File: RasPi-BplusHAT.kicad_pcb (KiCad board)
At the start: 2 copper layers, 65 x 56 mm, 11 parts, among them K1 PIN20X2, U1 EEPROM24

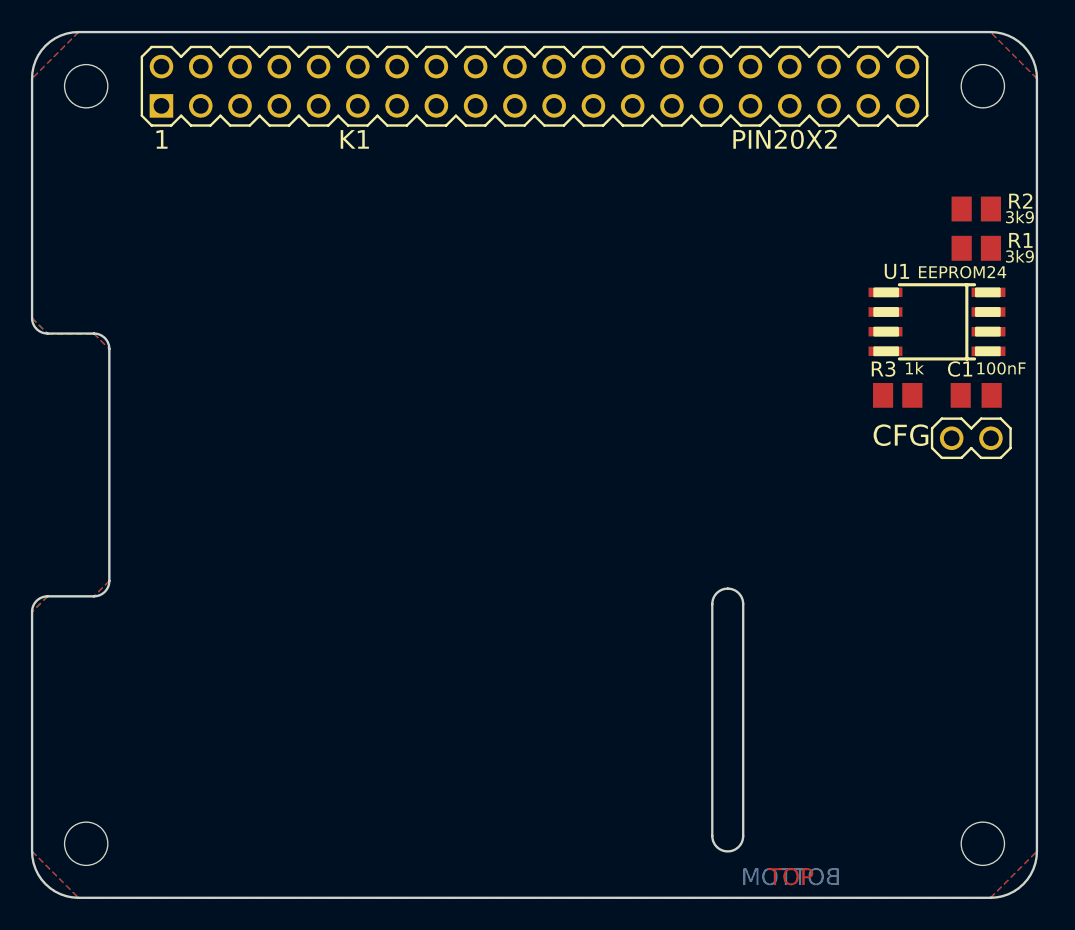
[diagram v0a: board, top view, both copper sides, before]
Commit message: Fix zones
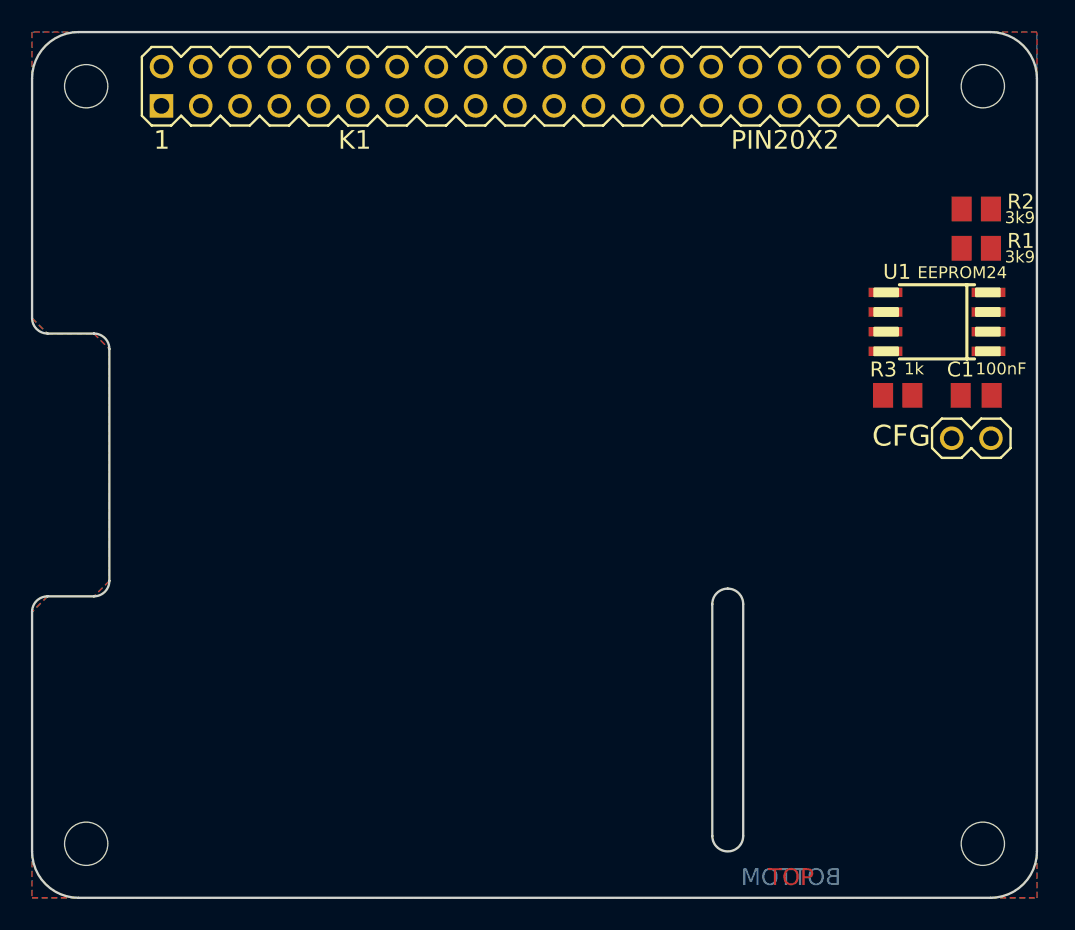
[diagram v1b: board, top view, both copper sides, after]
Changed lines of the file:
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@@
     (links 26)
     (no_connects 26)
-    (area 114.665415 76.924999 182.336786 133.075001)
+    (area 115.924999 76.924999 181.075001 133.075001)
     (thickness 1.6)
     (drawings 23)
@@
   (page A4)
   (layers
-    (0 Top signal hide)
-    (31 Bottom signal hide)
+    (0 Top signal)
+    (31 Bottom signal)
     (32 B.Adhes user)
     (33 F.Adhes user)
@@
     (42 Eco1.User user)
     (43 Eco2.User user)
-    (44 Edge.Cuts user)
+    (44 Edge.Cuts user hide)
     (45 Margin user)
     (46 B.CrtYd user)
@@
     (connect_pads (clearance 0.508))
     (min_thickness 0.254)
-    (fill (arc_segments 32) (thermal_gap 0.508) (thermal_bridge_width 0.508))
+    (fill yes (arc_segments 32) (thermal_gap 0.508) (thermal_bridge_width 0.508))
     (polygon
       (pts
-        (xy 116.0011 130.0036) (xy 119.0011 133.0036) (xy 178.0011 133.0036) (xy 181.0011 130.0036) (xy 181.0011 80.0036)
-        (xy 178.0011 77.0036) (xy 119.0011 77.0036) (xy 116.0011 80.0036) (xy 116.0011 95.5036) (xy 117.0011 96.5036)
+        (xy 116.0011 130.0036) (xy 116 133) (xy 178.0011 133.0036) (xy 181 133) (xy 181.0011 80.0036)
+        (xy 181 77) (xy 116 77) (xy 116.0011 80.0036) (xy 116.0011 95.5036) (xy 117.0011 96.5036)
         (xy 120.0011 96.5036) (xy 121.0011 97.5036) (xy 121.0011 112.5036) (xy 120.0011 113.5036) (xy 117.0011 113.5036)
         (xy 116.0011 114.5036)
@@
     (connect_pads (clearance 0.508))
     (min_thickness 0.254)
-    (fill (arc_segments 32) (thermal_gap 0.508) (thermal_bridge_width 0.508))
+    (fill yes (arc_segments 32) (thermal_gap 0.508) (thermal_bridge_width 0.508))
     (polygon
       (pts
-        (xy 116.0011 130.0036) (xy 119.0011 133.0036) (xy 178.0011 133.0036) (xy 181.0011 130.0036) (xy 181.0011 80.0036)
-        (xy 178.0011 77.0036) (xy 119.0011 77.0036) (xy 116.0011 80.0036) (xy 116.0011 95.5036) (xy 117.0011 96.5036)
+        (xy 116 133) (xy 119.0011 133.0036) (xy 181 133) (xy 181 130) (xy 181 77)
+        (xy 178.0011 77.0036) (xy 119.0011 77.0036) (xy 116 77) (xy 116.0011 95.5036) (xy 117.0011 96.5036)
         (xy 120.0011 96.5036) (xy 121.0011 97.5036) (xy 121.0011 112.5036) (xy 120.0011 113.5036) (xy 117.0011 113.5036)
         (xy 116.0011 114.5036)
